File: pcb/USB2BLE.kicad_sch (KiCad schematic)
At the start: 10 parts, among them J1 Conn_01x02, SW1 SW_SPDT, U1 XIAO-ESP32-S3-SMD, U2 MT3608

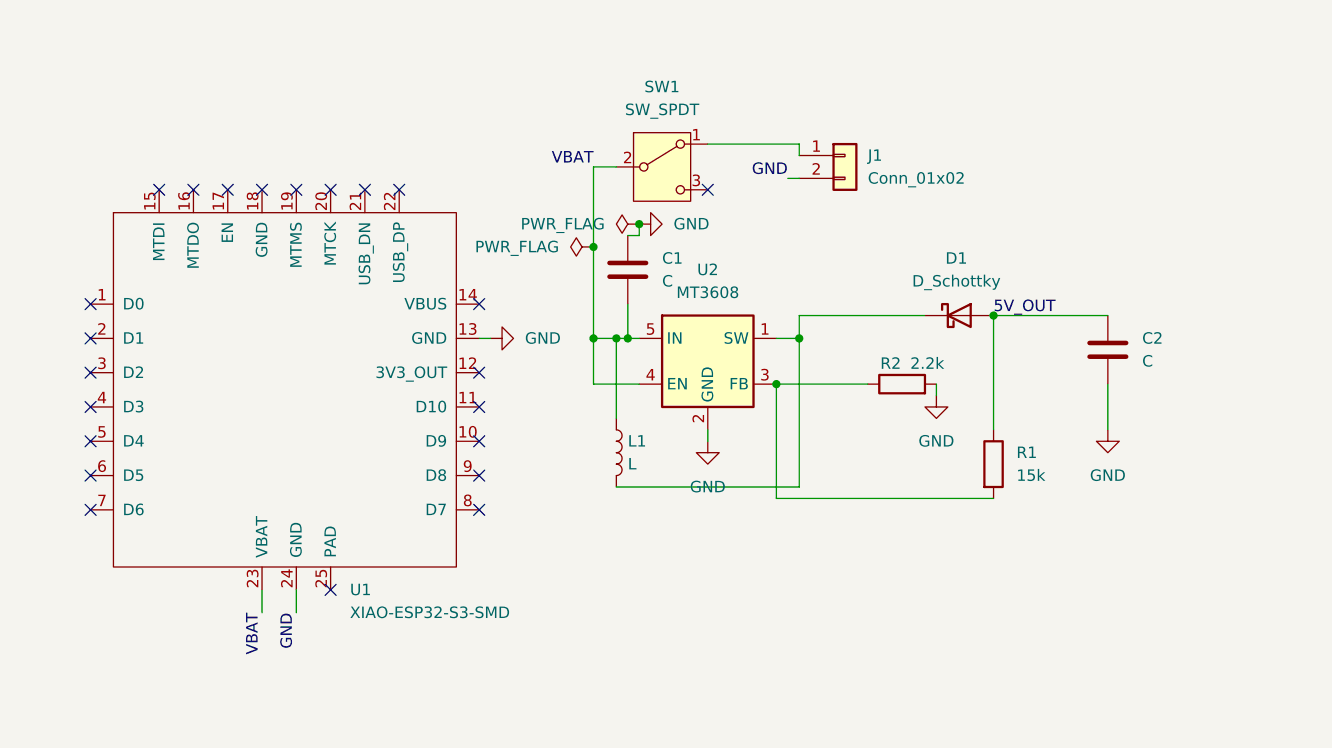
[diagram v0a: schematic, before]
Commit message: updated
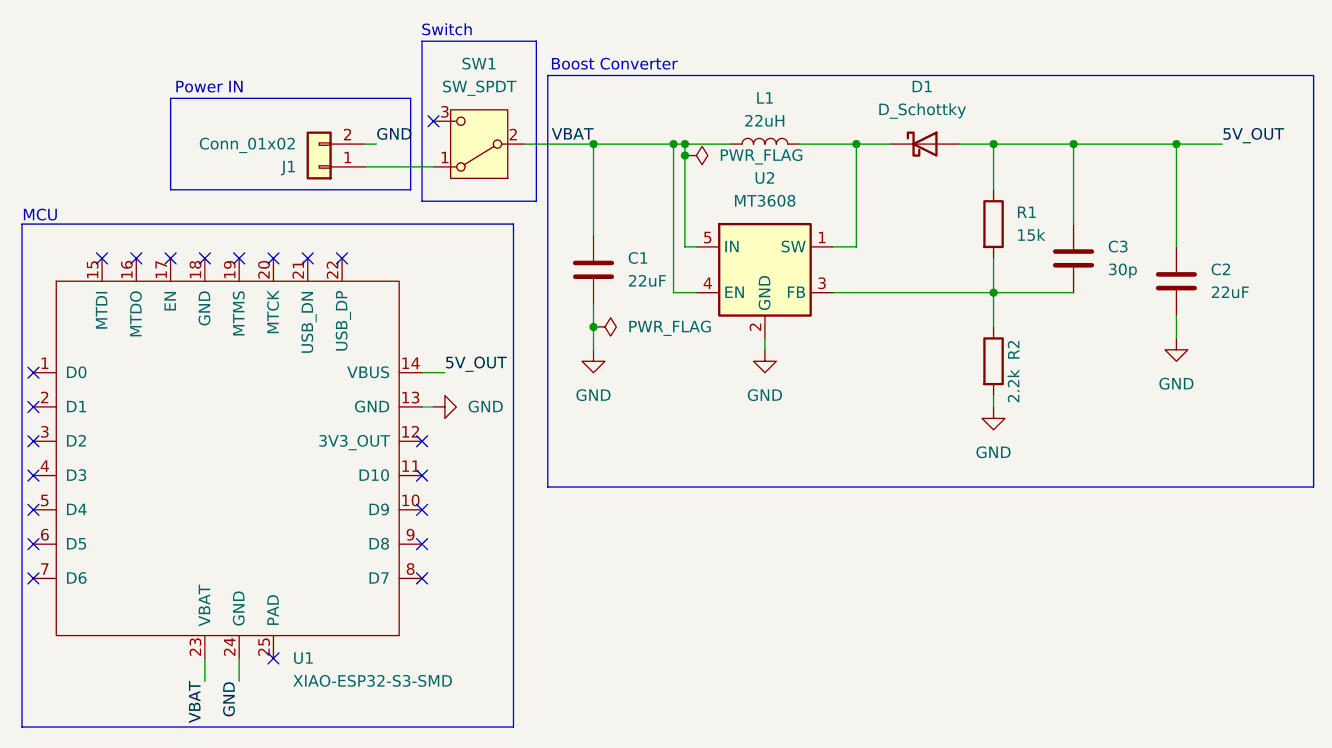
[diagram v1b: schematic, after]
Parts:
- added C3: 30p, Capacitor_SMD:C_0805_2012Metric_Pad1.18x1.45mm_HandSolder, symbol Device:C
- C1, C2: value C -> 22uF
- L1: value L -> 22uH
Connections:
- net 5V_OUT: now also U1.14 (VBUS), C3.1
- net GND: now also C1.2; no longer C1.1
- net VBAT: now also C1.1; no longer C1.2
- net at R1.2, R2.1, U2.3 (FB): now also C3.2
- no-connect marks 23 -> 22
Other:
- note added: "Boost Converter"
- note added: "MCU"
- note added: "Power IN"
- note added: "Switch"
- moved on the sheet: C1, C2, D1, J1, L1, R1, R2, SW1, U1, U2
